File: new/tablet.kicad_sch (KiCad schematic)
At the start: 49 parts, among them J1 FSMC/TOUCH-SPI, J2 USB_B_Micro, J3 SD/CARD, J4 FLASH/FONT, J5 Conn_02x03_Odd_Even, J6 Conn_01x02, J7 Conn_ARM_SWD_TagConnect_TC2030, Q1 DMG2301L, SW1 SW_SPST, U1 STM32F429Z_E-G_Tx, U2 TPS63001, U3 MCP73811T-420I-OT, Y1 Crystal

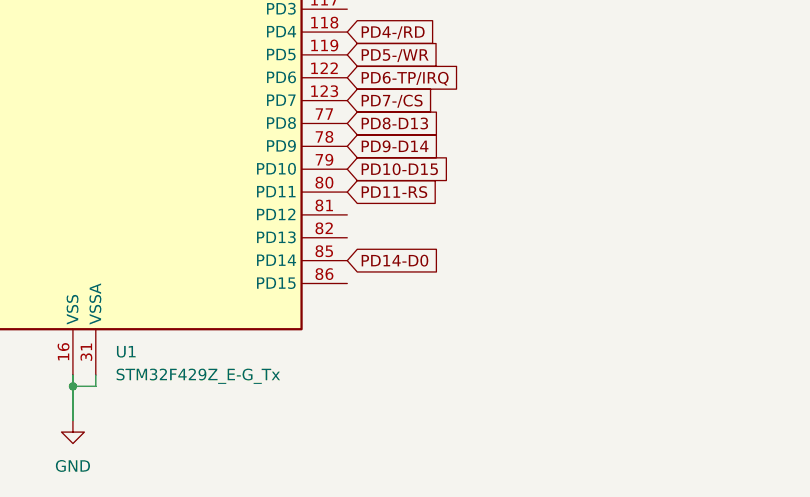
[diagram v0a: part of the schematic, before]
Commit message: send for production
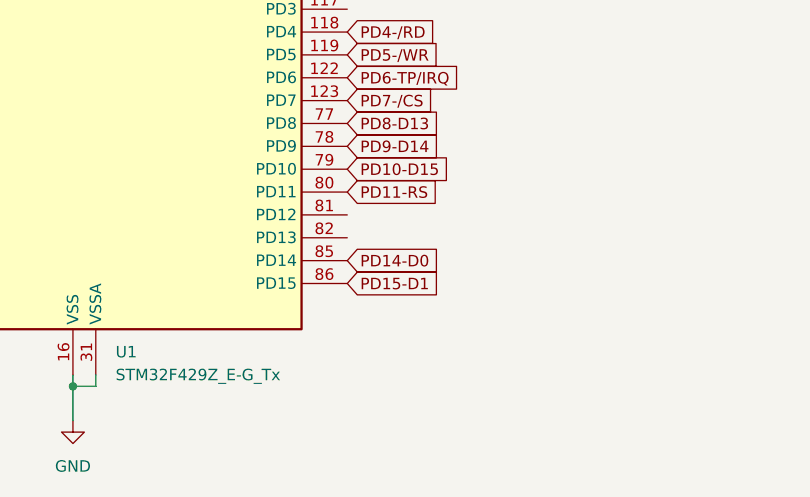
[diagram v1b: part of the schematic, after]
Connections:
- net PD15-D1: now also U1.86 (PD15)
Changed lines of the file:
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@@
+    )
+  )
+  (global_label "PD15-D1" (shape input) (at 139.7 247.65 0) (fields_autoplaced)
+    (effects (font (size 1.27 1.27)) (justify left))
+    (property "Intersheetrefs" "${INTERSHEET_REFS}" (at 151.6961 247.65 0)
+      (effects (font (size 1.27 1.27)) (justify left) hide)
     )
   )
